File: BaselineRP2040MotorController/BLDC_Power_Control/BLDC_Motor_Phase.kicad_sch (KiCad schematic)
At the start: 30 parts, among them Q3 Q_PNP_BEC, U10 INA240A1D, U9 EG3113

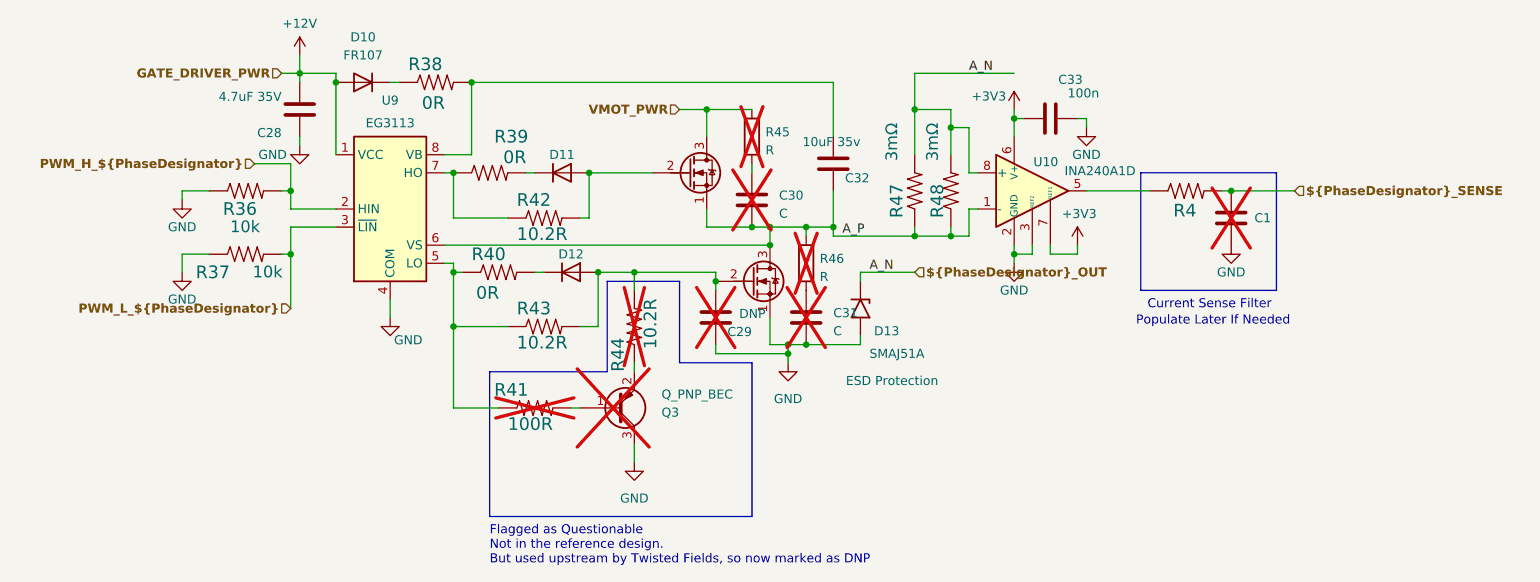
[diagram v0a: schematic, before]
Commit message: MinMax
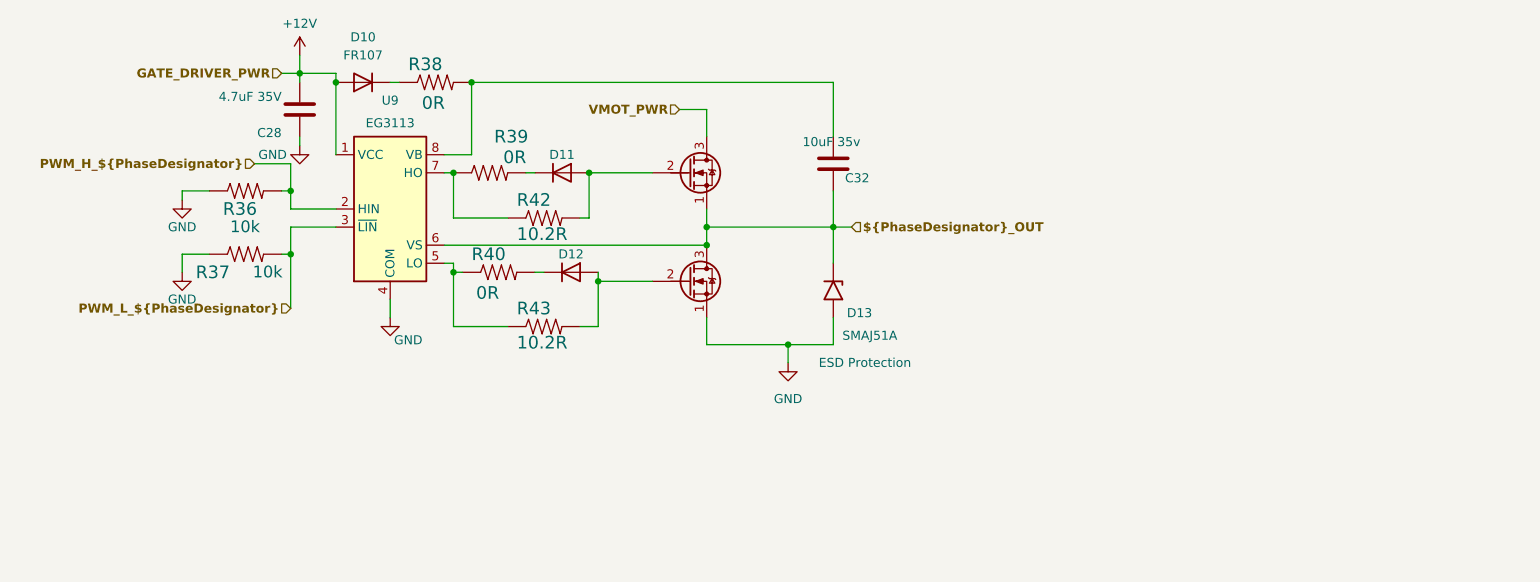
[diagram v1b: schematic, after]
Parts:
- removed C1: 0, Capacitor_SMD:C_0603_1608Metric, symbol Device:C
- removed C29: DNP, Capacitor_SMD:C_0603_1608Metric, symbol Device:C
- removed C30, C31: C, Capacitor_SMD:C_0805_2012Metric, symbol Device:C
- removed C33: 100n, Capacitor_SMD:C_0603_1608Metric, symbol Device:C
- removed Q3: Q_PNP_BEC, Package_TO_SOT_SMD:SOT-23, symbol Device:Q_PNP_BEC
- removed R4: 0, Resistor_SMD:R_0603_1608Metric, symbol MotorController:TAYLOR_RESISTOR
- removed R41: 100R, Resistor_SMD:R_0603_1608Metric, symbol MotorController:TAYLOR_RESISTOR
- removed R44: 10.2R, Resistor_SMD:R_0603_1608Metric, symbol MotorController:TAYLOR_RESISTOR
- removed R45, R46: R, Resistor_SMD:R_0805_2012Metric, symbol Device:R
- removed R47, R48: 3mΩ, Resistor_SMD:R_2512_6332Metric, symbol MotorController:TAYLOR_RESISTOR
- removed U10: INA240A1D, Package_SO:SOIC-8_3.9x4.9mm_P1.27mm, symbol Amplifier_Current:INA240A1D
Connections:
- net A_P is gone; now on net ${PhaseDesignator}_OUT: AH3.1 (S), AL3.3 (D), C32.1, U9.6 (VS)
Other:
- note removed: "Current Sense Filter"
- note removed: "Flagged as Questionable Not in the reference design. But used upstream by Twisted Fields, so now marked as DNP"
- note removed: "Populate Later If Needed"
- moved on the sheet: D13
